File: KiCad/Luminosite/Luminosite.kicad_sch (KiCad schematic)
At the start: 1 part, among them U4 ESP32-C3_SUPERMINI_TH

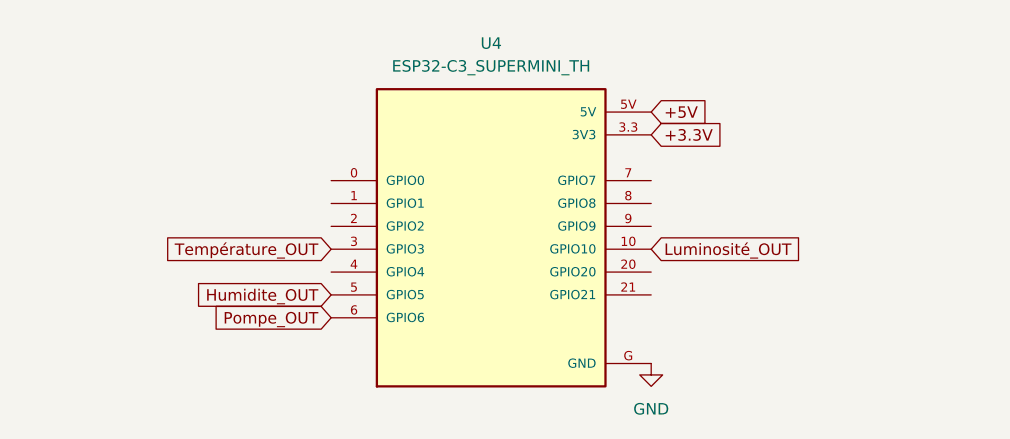
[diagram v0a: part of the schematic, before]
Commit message: PCB Terminé
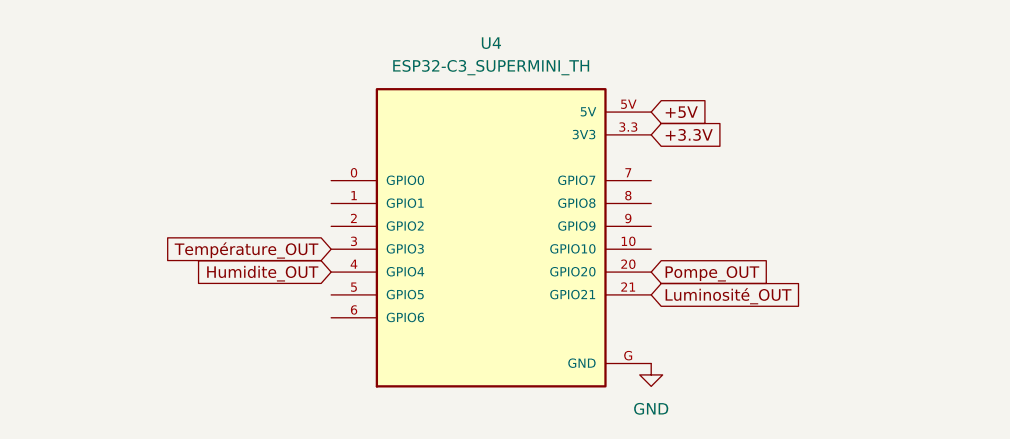
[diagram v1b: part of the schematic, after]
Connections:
- net Humidite_OUT: now also U4.4 (GPIO4); no longer U4.5 (GPIO5)
- net Luminosité_OUT: now also U4.21 (GPIO21); no longer U4.10 (GPIO10)
- net Pompe_OUT: now also U4.20 (GPIO20); no longer U4.6 (GPIO6)
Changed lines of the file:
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@@
 	(generator_version "10.0")
 	(paper "A4")
+	(global_label "Luminosité_OUT"
+		(shape input)
+		(at 139.7 121.92 0)
+		(fields_autoplaced yes)
+		(effects
+			(font
+				(size 1.27 1.27)
+			)
+			(justify left)
+		)
+		(property "Intersheetrefs" "${INTERSHEET_REFS}"
+			(at 156.8476 121.92 0)
+			(hide yes)
+			(show_name no)
+			(do_not_autoplace no)
+			(effects
+				(font
+					(size 1.27 1.27)
+				)
+				(justify left)
+			)
+		)
+	)
 	(global_label "Température_OUT"
 		(shape input)
@@
 		(property "Intersheetrefs" "${INTERSHEET_REFS}"
 			(at 85.541 116.84 0)
-			(hide yes)
-			(show_name no)
-			(do_not_autoplace no)
-			(effects
-				(font
-					(size 1.27 1.27)
-				)
-				(justify right)
-			)
-		)
-	)
-	(global_label "Pompe_OUT"
-		(shape input)
-		(at 104.14 124.46 180)
-		(fields_autoplaced yes)
-		(effects
-			(font
-				(size 1.27 1.27)
-			)
-			(justify right)
-		)
-		(property "Intersheetrefs" "${INTERSHEET_REFS}"
-			(at 90.8629 124.46 0)
 			(hide yes)
 			(show_name no)
@@
 		)
 	)
-	(global_label "Luminosité_OUT"
+	(global_label "Humidite_OUT"
 		(shape input)
-		(at 139.7 116.84 0)
+		(at 104.14 119.38 180)
+		(fields_autoplaced yes)
+		(effects
+			(font
+				(size 1.27 1.27)
+			)
+			(justify right)
+		)
+		(property "Intersheetrefs" "${INTERSHEET_REFS}"
+			(at 88.8671 119.38 0)
+			(hide yes)
+			(show_name no)
+			(do_not_autoplace no)
+			(effects
+				(font
+					(size 1.27 1.27)
+				)
+				(justify right)
+			)
+		)
+	)
+	(global_label "Pompe_OUT"
+		(shape input)
+		(at 139.7 119.38 0)
 		(fields_autoplaced yes)
 		(effects
@@
 		)
 		(property "Intersheetrefs" "${INTERSHEET_REFS}"
-			(at 156.8476 116.84 0)
+			(at 152.9771 119.38 0)
 			(hide yes)
 			(show_name no)
@@
 			)
 		)
-	)
-	(global_label "Humidite_OUT"
-		(shape input)
-		(at 104.14 121.92 180)
-		(fields_autoplaced yes)
-		(effects
-			(font
-				(size 1.27 1.27)
-			)
-			(justify right)
-		)
-		(property "Intersheetrefs" "${INTERSHEET_REFS}"
-			(at 88.8671 121.92 0)
-			(hide yes)
-			(show_name no)
-			(do_not_autoplace no)
-			(effects
-				(font
-					(size 1.27 1.27)
-				)
-				(justify right)
-			)
-		)
